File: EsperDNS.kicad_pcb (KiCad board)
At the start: 2 copper layers, 147.7 x 110.7 mm, 61 parts, among them J1 10118192-0001LF, J2 ARJM11A3, J3 Conn_02x05_Odd_Even, Q1 Q_NMOS_GSD, Q2 Q_NMOS_GSD, Q3 Q_NMOS_GSD, SW1 222CMVBAR, SW2 222CMVBAR, U1 AZ1117-3.3, U2 LAN8720A, U3 ESP32-WROOM-32D, X1 ECS-2520MV

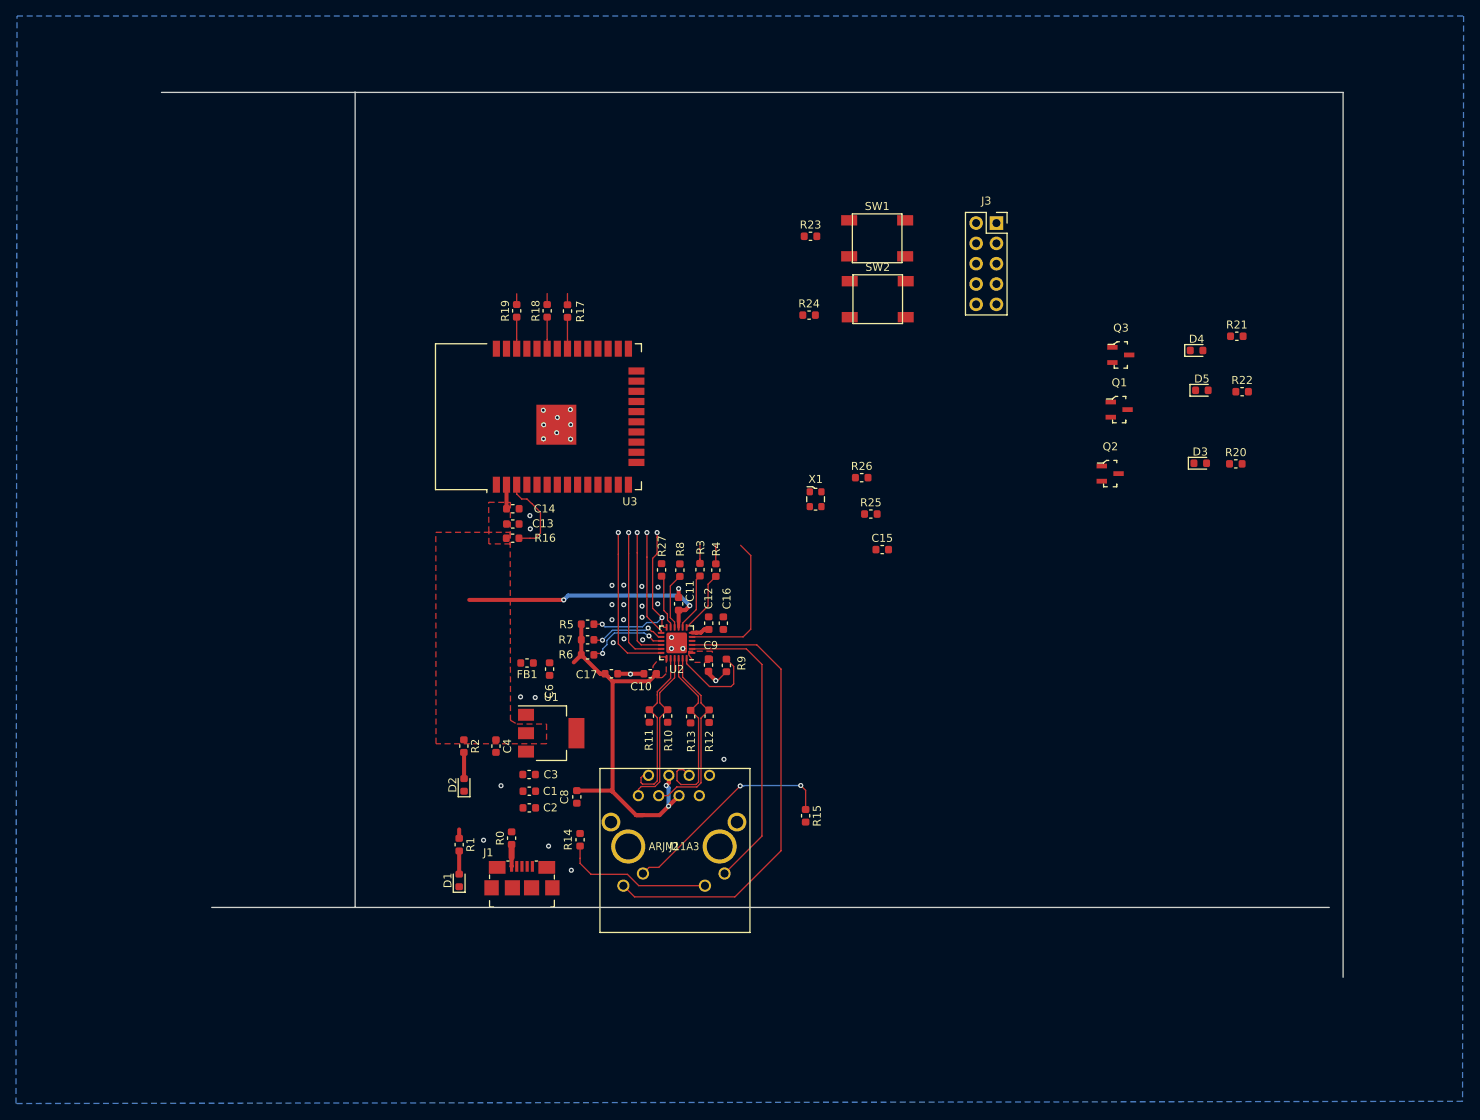
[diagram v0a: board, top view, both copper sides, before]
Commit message: Worked on board
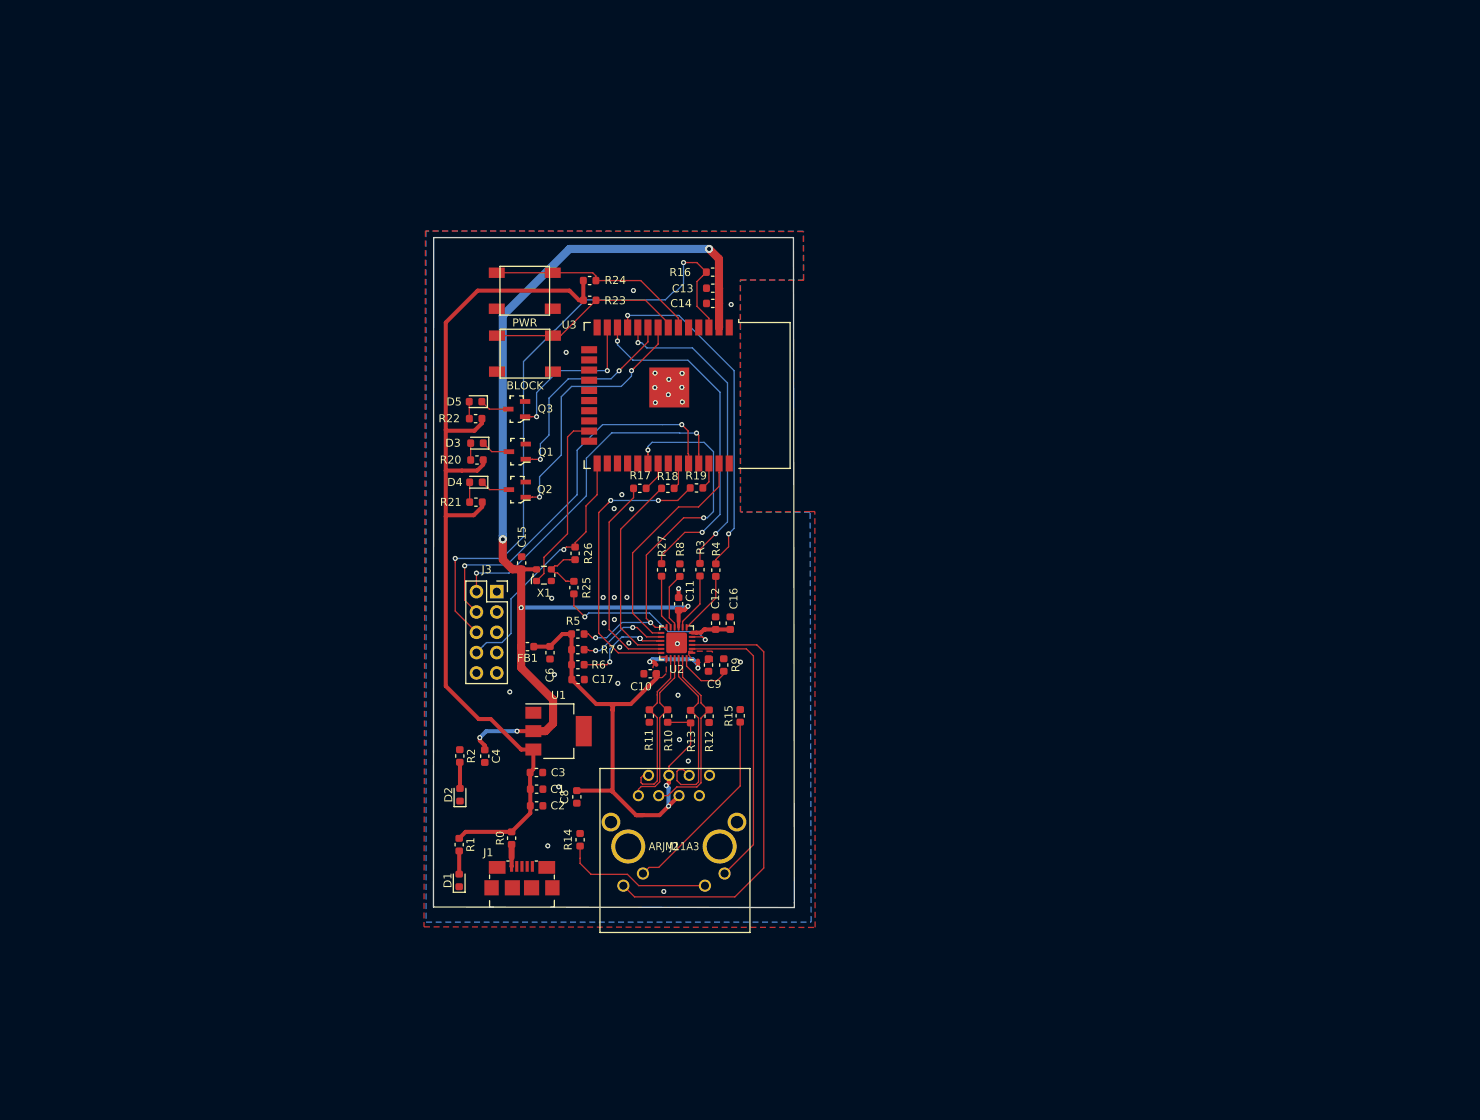
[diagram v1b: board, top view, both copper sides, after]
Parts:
- moved R21 97.3 mm to (121.9, 89.0), turned to 180 degrees
- moved R22 95.9 mm to (121.9, 78.6), turned to 180 degrees
- moved R20 94.9 mm to (122.1, 83.8), turned to 180 degrees
- moved D4 91.6 mm to (121.9, 86.6), turned to 180 degrees
- moved D5 90.8 mm to (121.9, 76.5), turned to 180 degrees
- moved D3 90.4 mm to (122.1, 81.7), turned to 180 degrees
- moved J3 77.6 mm to (124.5, 100.2)
- moved Q3 75.8 mm to (127.0, 77.4), turned to 180 degrees
- moved Q1 75.4 mm to (127.1, 82.7), turned to 180 degrees
- moved Q2 74.1 mm to (127.1, 87.5), turned to 180 degrees
- moved BLOCK 46.3 mm to (128.1, 70.5), turned to 180 degrees
- moved C15 45.1 mm to (127.6, 96.6), turned to 270 degrees
- moved PWR 44.1 mm to (128.0, 62.6), turned to 180 degrees
- moved R16 41.6 mm to (151.5, 60.3), turned to 0 degrees
- moved C13 38.6 mm to (151.5, 62.3), turned to 0 degrees
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- renumbered SW1 to BLOCK, SW2 to PWR
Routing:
- net VBUS: track 1.19 -> 116.8 mm
- net +3V3: track 35.2 -> 131.9 mm, vias 2 -> 6
- net EN: track 10.6 -> 79.9 mm, vias 0 -> 2
- net RX: track 0.00 -> 49.3 mm, vias 0 -> 2
- net TX: track 0.00 -> 43.8 mm, vias 0 -> 2
- net CRS_DV: track 6.86 -> 50.0 mm, vias 0 -> 2
- net RXD1: track 2.36 -> 42.8 mm, vias 0 -> 2
- net RXD0: track 2.39 -> 39.2 mm, vias 0 -> 2
- net RED: track 0.00 -> 32.7 mm, vias 0 -> 2
- net BOOTMODE: track 0.00 -> 31.9 mm, vias 0 -> 1
- net MDIO: track 22.1 -> 49.4 mm, vias 3 -> 4
- net YELLOW: track 0.00 -> 27.0 mm, vias 0 -> 2
- net RESTART: track 0.00 -> 26.6 mm
- net AVDD: track 50.2 -> 76.0 mm, vias 2 -> 4
- net BLOCK: track 0.00 -> 25.0 mm
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- added copper zone on F.Cu, net GND
- removed copper zone on F.Cu, net +3V3
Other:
- board size 147.7 x 110.7 mm -> 45.1 x 83.7 mm
